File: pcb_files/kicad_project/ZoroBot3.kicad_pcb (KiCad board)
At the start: 2 copper layers, 67.6 x 110.7 mm, 175 parts, among them Q1 NMOS, Q2 AON7423, Q3 ST-1KL3A, Q4 ST-1KL3A, Q5 ST-1KL3A, Q6 ST-1KL3A, U1 MPU-6500, U2 MPU-6500, Y1 Crystal_GND24

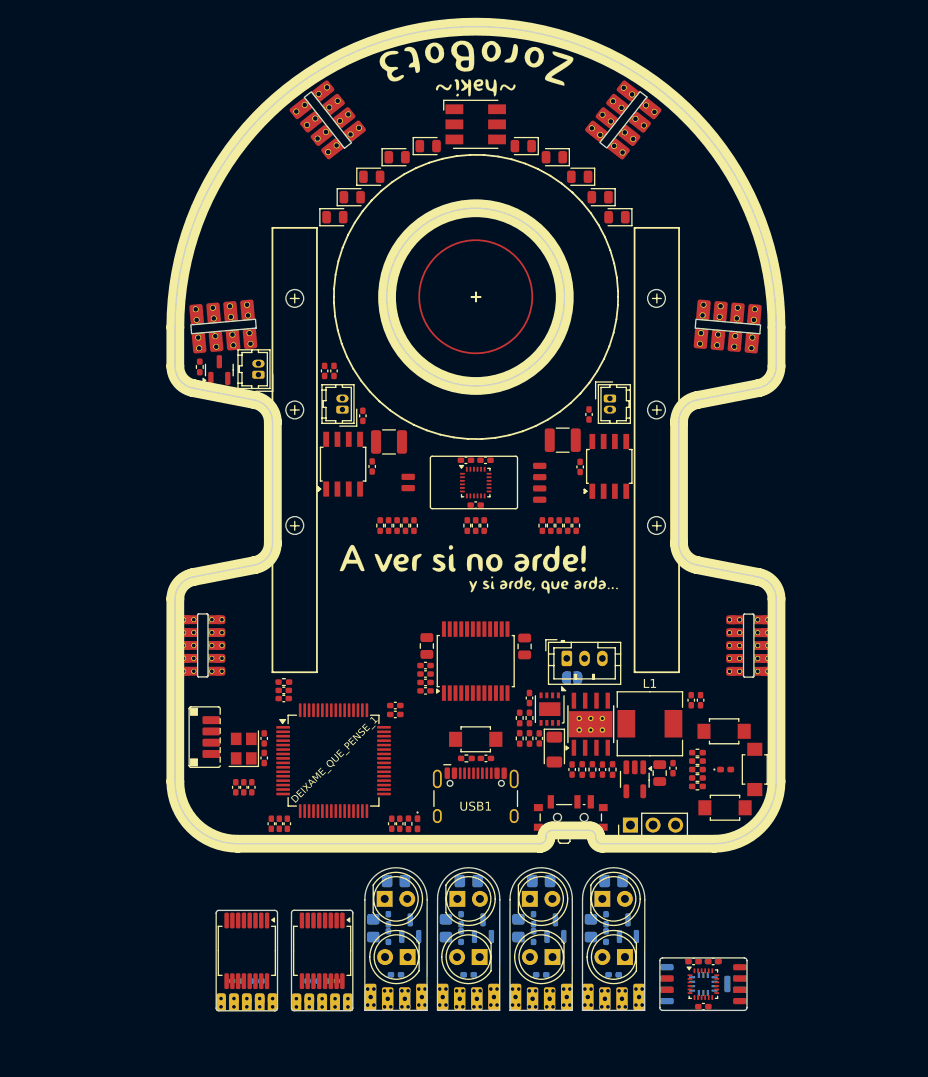
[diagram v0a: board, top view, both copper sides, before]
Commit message: Finaliza el diseño de la PCB de ZoroBot3 Rebuild y añade gerbers y BOM
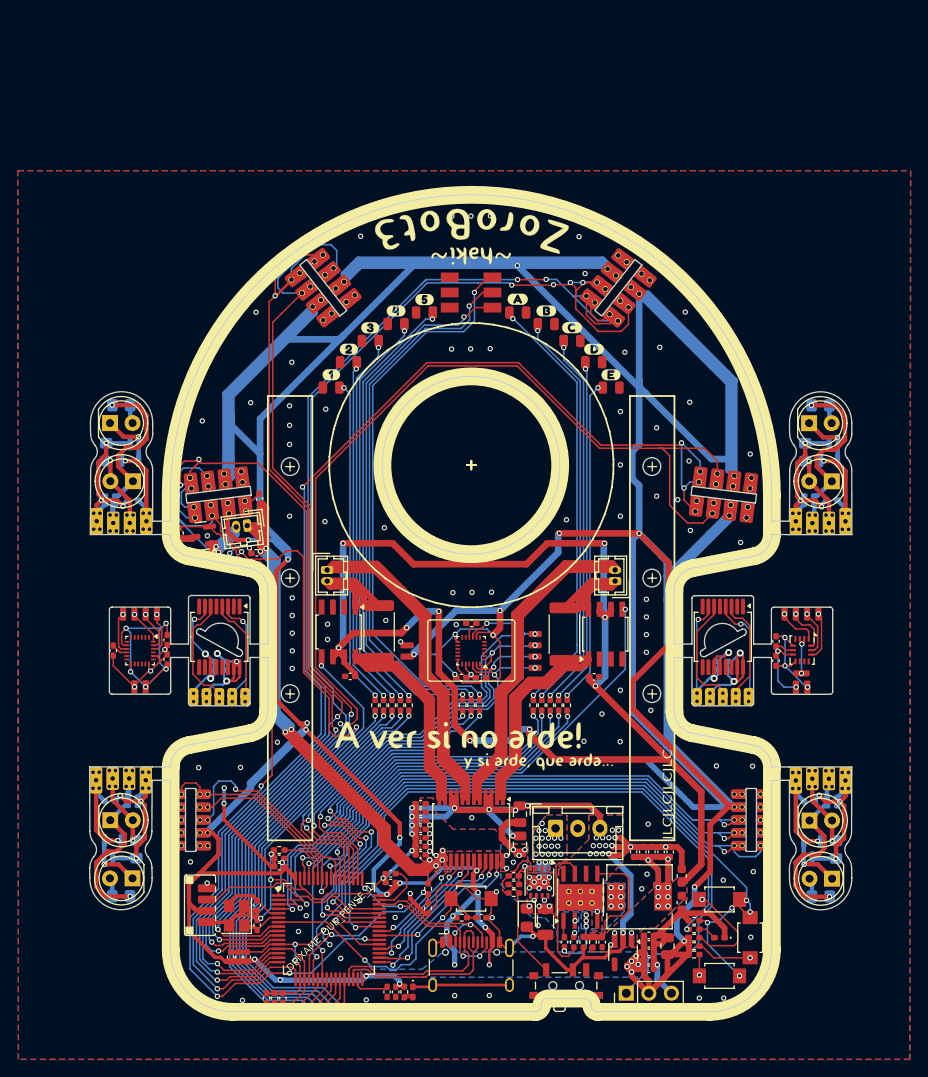
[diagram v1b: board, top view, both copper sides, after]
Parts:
- removed C14, C16: 0.1uF, Capacitor_SMD:C_0402_1005Metric_Pad0.74x0.62mm_HandSolder
- added C41: 10uF, Capacitor_SMD:C_0402_1005Metric_Pad0.74x0.62mm_HandSolder, F.Cu at (144.9, 119.4)
- added C42: 10uF, Capacitor_SMD:C_0402_1005Metric_Pad0.74x0.62mm_HandSolder, F.Cu at (144.9, 120.4)
- added C43: 10uF, Capacitor_SMD:C_0402_1005Metric_Pad0.74x0.62mm_HandSolder, F.Cu at (144.9, 121.4)
- added C44: 10uF, Capacitor_SMD:C_0402_1005Metric_Pad0.74x0.62mm_HandSolder, F.Cu at (170.6, 137.1)
- added C45: 10uF, Capacitor_SMD:C_0402_1005Metric_Pad0.74x0.62mm_HandSolder, F.Cu at (170.6, 135.2)
- added C46: 10uF, Capacitor_SMD:C_0402_1005Metric_Pad0.74x0.62mm_HandSolder, F.Cu at (170.6, 136.2)
- added C47: 10uF, Capacitor_SMD:C_0402_1005Metric_Pad0.74x0.62mm_HandSolder, F.Cu at (173.0, 124.9)
- added C48: 10uF, Capacitor_SMD:C_0402_1005Metric_Pad0.74x0.62mm_HandSolder, F.Cu at (170.9, 124.9)
- added C49: 10uF, Capacitor_SMD:C_0402_1005Metric_Pad0.74x0.62mm_HandSolder, F.Cu at (172.0, 124.9)
- added C50: 10uF, Capacitor_SMD:C_0402_1005Metric_Pad0.74x0.62mm_HandSolder, F.Cu at (168.9, 124.9)
- added C51: 10uF, Capacitor_SMD:C_0402_1005Metric_Pad0.74x0.62mm_HandSolder, F.Cu at (169.9, 124.9)
- added C52: 10uF, Capacitor_SMD:C_0402_1005Metric_Pad0.74x0.62mm_HandSolder, F.Cu at (170.6, 138.1)
- added kibuzzard-6779A98A: G***, kibuzzard-6779A98A, B.Cu at (110.8, 99.0)
- added kibuzzard-6779A9B1: G***, kibuzzard-6779A9B1, B.Cu at (185.3, 98.9)
- added kibuzzard-677A7C8F: G***, kibuzzard-677A7C8F, F.Cu at (155.8, 62.7)
- added kibuzzard-677A7C9A: G***, kibuzzard-677A7C9A, F.Cu at (159.0, 64.0)
- added kibuzzard-677A7CA3: G***, kibuzzard-677A7CA3, F.Cu at (161.9, 65.9)
- added kibuzzard-677A7CAF: G***, kibuzzard-677A7CAF, F.Cu at (164.4, 68.3)
- added kibuzzard-677A7CBB: G***, kibuzzard-677A7CBB, F.Cu at (166.3, 71.2)
- added kibuzzard-677A7D71: G***, kibuzzard-677A7D71, F.Cu at (136.8, 68.3)
- added kibuzzard-677A7D7B: G***, kibuzzard-677A7D7B, F.Cu at (139.2, 65.9)
- added kibuzzard-677A7D86: G***, kibuzzard-677A7D86, F.Cu at (142.1, 64.0)
- added kibuzzard-677A7E2E: G***, kibuzzard-677A7E2E, F.Cu at (134.8, 71.2)
- added kibuzzard-677A7E3B: G***, kibuzzard-677A7E3B, F.Cu at (145.3, 62.7)
- AS5145B_D1, AS5145B_I1: footprint Package_SO:SSOP-16_5.3x6.2mm_P0.65mm -> custom_footprints:Encoder_AS5145B
- BATT1: footprint Connector_JST:JST_PH_B3B-PH-K_1x03_P2.00mm_Vertical -> Connector_JST:JST_XH_B3B-XH-A_1x03_P2.50mm_Vertical
- C37, C38, DATA_MPU2, JP3, LSM6DSR1, POWER_MPU3: moved to F.Cu
- CR4, CR7: footprint Capacitor_SMD:C_0402_1005Metric_Pad0.74x0.62mm_HandSolder -> Capacitor_SMD:C_0603_1608Metric
- CR6: value 0.1uF -> 47uF; footprint Capacitor_SMD:C_0402_1005Metric_Pad0.74x0.62mm_HandSolder -> Capacitor_SMD:C_1206_3216Metric
- D13: footprint Diode_SMD:D_1206_3216Metric -> Diode_SMD:D_0805_2012Metric_Pad1.15x1.40mm_HandSolder
- MOSFET-N1, MOSFET-N2, MOSFET-N3, MOSFET-N4: value AO3401 -> AO3400 (A09T)
- R12, R13: footprint Resistor_SMD:R_1210_3225Metric -> Resistor_SMD:R_2512_6332Metric
- moved DATA_MPU3 79.3 mm to (113.3, 98.1), turned to 90 degrees
- moved C40 77.5 mm to (110.3, 102.2), turned to 90 degrees
- moved POWER_MPU3 75.3 mm to (113.3, 106.3), turned to 90 degrees
- moved U2 73.7 mm to (113.3, 102.2), turned to -90 degrees
- moved C39 71.3 mm to (116.4, 101.0), turned to 90 degrees
- moved C36 68.3 mm to (116.4, 103.2), turned to -90 degrees
- moved C33 65.4 mm to (178.9, 103.4), turned to 180 degrees
- moved AS5145B_D1 64.2 mm to (178.9, 100.7)
- moved ENC_D_CONN1 63.6 mm to (178.9, 106.3)
- moved C32 63.1 mm to (178.9, 104.4)
- moved RS9 62.5 mm to (188.2, 79.9)
- moved CONN_SEN_PA_I1 62.3 mm to (111.2, 87.8)
- moved MOSFET-N2 62.2 mm to (112.2, 79.9)
- moved LED_IR3 62.1 mm to (188.6, 76.6)
- moved RS7 62.1 mm to (189.9, 74.6)
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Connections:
- AD8418AWBZ_2 pad 1: /SHUNT_MI -> /MOT_I-
- AD8418AWBZ_2 pad 8: /MOT_I+ -> /SHUNT_MI
- C36 pad 1: /Giroscopio/GND_MPU -> /Giroscopio/GND_MPU_A
- C36 pad 2: /Giroscopio/3.3_MPU -> /Giroscopio/3.3_MPU_A
- C37 pad 1: /Giroscopio/GND_MPU -> /Giroscopio/GND_MPU_B
- C37 pad 2: /Giroscopio/3.3_MPU -> /Giroscopio/3.3_MPU_B
- C38 pad 1: /Giroscopio/GND_MPU -> /Giroscopio/GND_MPU_B
- C38 pad 2: /Giroscopio/3.3_MPU -> /Giroscopio/3.3_MPU_B
- C39 pad 1: /Giroscopio/GND_MPU -> /Giroscopio/GND_MPU_A
- C39 pad 2: /Giroscopio/3.3_MPU -> /Giroscopio/3.3_MPU_A
- C40 pad 1: /Giroscopio/GND_MPU -> /Giroscopio/GND_MPU_A
- DATA_MPU2 pad 1: /Giroscopio/SPI_MISO_CONN -> /Giroscopio/SPI_MISO_CONN_B
- DATA_MPU2 pad 2: /Giroscopio/SPI_MOSI_CONN -> /Giroscopio/SPI_MOSI_CONN_B
- DATA_MPU2 pad 3: /Giroscopio/SPI_SCK_CONN -> /Giroscopio/SPI_SCK_CONN_B
- DATA_MPU2 pad 4: /Giroscopio/SPI_NSS_CONN -> /Giroscopio/SPI_NSS_CONN_B
- DATA_MPU3 pad 1: /Giroscopio/SPI_MISO_CONN -> /Giroscopio/SPI_MISO_CONN_A
- DATA_MPU3 pad 2: /Giroscopio/SPI_MOSI_CONN -> /Giroscopio/SPI_MOSI_CONN_A
- DATA_MPU3 pad 3: /Giroscopio/SPI_SCK_CONN -> /Giroscopio/SPI_SCK_CONN_A
- DATA_MPU3 pad 4: /Giroscopio/SPI_NSS_CONN -> /Giroscopio/SPI_NSS_CONN_A
- DEIXAME_QUE_PENSE_1 pad 54: /ENC_2_I -> /ENC_D_I
- DEIXAME_QUE_PENSE_1 pad 55: /ENC_1_I -> /ENC_I_I
- DEIXAME_QUE_PENSE_1 pad 56: /ENC_2_B -> /ENC_D_B
- DEIXAME_QUE_PENSE_1 pad 57: /ENC_2_A -> /ENC_D_A
- DEIXAME_QUE_PENSE_1 pad 58: /ENC_1_B -> /ENC_I_B
- DEIXAME_QUE_PENSE_1 pad 59: /ENC_1_A -> /ENC_I_A
- ENC_D1 pad 3: /ENC_1_A -> /ENC_D_I
- ENC_D1 pad 4: /ENC_1_B -> /ENC_D_A
- ENC_D1 pad 5: /ENC_1_I -> /ENC_D_B
- ENC_D_CONN1 pad 3: /Encoders/ENC_D_A_CONN -> /Encoders/ENC_D_I_CONN
- ENC_D_CONN1 pad 4: /Encoders/ENC_D_B_CONN -> /Encoders/ENC_D_A_CONN
- ENC_D_CONN1 pad 5: /Encoders/ENC_D_I_CONN -> /Encoders/ENC_D_B_CONN
- ENC_I1 pad 3: /ENC_2_A -> /ENC_I_I
- ENC_I1 pad 4: /ENC_2_B -> /ENC_I_A
- ENC_I1 pad 5: /ENC_2_I -> /ENC_I_B
- ENC_I_CONN1 pad 3: /Encoders/ENC_I_A_CONN -> /Encoders/ENC_I_I_CONN
- ENC_I_CONN1 pad 4: /Encoders/ENC_I_B_CONN -> /Encoders/ENC_I_A_CONN
- ENC_I_CONN1 pad 5: /Encoders/ENC_I_I_CONN -> /Encoders/ENC_I_B_CONN
- LSM6DSR1 pad 1: /Giroscopio/SPI_MISO_CONN -> /Giroscopio/SPI_MISO_CONN_B
- LSM6DSR1 pad 12: /Giroscopio/SPI_NSS_CONN -> /Giroscopio/SPI_NSS_CONN_B
- LSM6DSR1 pad 13: /Giroscopio/SPI_SCK_CONN -> /Giroscopio/SPI_SCK_CONN_B
- LSM6DSR1 pad 14: /Giroscopio/SPI_MOSI_CONN -> /Giroscopio/SPI_MOSI_CONN_B
- LSM6DSR1 pad 5: /Giroscopio/3.3_MPU -> /Giroscopio/3.3_MPU_B
- LSM6DSR1 pad 6: /Giroscopio/GND_MPU -> /Giroscopio/GND_MPU_B
- LSM6DSR1 pad 7: /Giroscopio/GND_MPU -> /Giroscopio/GND_MPU_B
- LSM6DSR1 pad 8: /Giroscopio/3.3_MPU -> /Giroscopio/3.3_MPU_B
- MOSFET-N1 pad 1: /Sensores/EMI_PA_D_CONN -> Net-(LED_IR1-K)
- MOSFET-N1 pad 2: /Sensores/GND_D -> /Sensores/EMI_PA_D_CONN
- MOSFET-N1 pad 3: Net-(LED_IR1-K) -> /Sensores/GND_D
- MOSFET-N2 pad 1: /Sensores/EMI_PA_I_CONN -> Net-(LED_IR2-K)
- MOSFET-N2 pad 2: /Sensores/GND_I -> /Sensores/EMI_PA_I_CONN
- MOSFET-N2 pad 3: Net-(LED_IR2-K) -> /Sensores/GND_I
- MOSFET-N3 pad 1: /Sensores/EMI_FRONT_D_CONN -> Net-(LED_IR3-K)
- MOSFET-N3 pad 2: /Sensores/GND_FD -> /Sensores/EMI_FRONT_D_CONN
- MOSFET-N3 pad 3: Net-(LED_IR3-K) -> /Sensores/GND_FD
- MOSFET-N4 pad 1: /Sensores/EMI_FRONT_I_CONN -> Net-(LED_IR4-K)
- MOSFET-N4 pad 2: /Sensores/GND_FI -> /Sensores/EMI_FRONT_I_CONN
- MOSFET-N4 pad 3: Net-(LED_IR4-K) -> /Sensores/GND_FI
- PH1 pad 1: /BATT -> /SHUNT_MD
- PH1 pad 10: /MOT_I_PWM -> GND
- PH1 pad 11: /BATT -> /SHUNT_MI
- PH1 pad 12: /BATT -> /SHUNT_MI
- PH1 pad 13: /SHUNT_MI -> /BATT
- PH1 pad 14: /SHUNT_MI -> /BATT
- PH1 pad 15: GND -> /MOT_I_PWM
- PH1 pad 16: GND -> /MOT_I_B
- PH1 pad 17: /MOT_I- -> /MOT_I_A
- PH1 pad 18: /MOT_I- -> GND
- PH1 pad 19: /MOT_D- -> +3V3
- PH1 pad 2: /MOT_D_PWM -> /SHUNT_MD
- PH1 pad 20: /MOT_D- -> +3V3
- PH1 pad 21: GND -> /MOT_D_B
- PH1 pad 22: GND -> /MOT_D_A
- PH1 pad 23: /SHUNT_MD -> /MOT_D_PWM
- PH1 pad 24: /SHUNT_MD -> /BATT
- PH1 pad 3: /MOT_D_A -> GND
- PH1 pad 4: /MOT_D_B -> GND
- PH1 pad 5: +3V3 -> /MOT_D-
- PH1 pad 6: +3V3 -> /MOT_D-
- PH1 pad 7: GND -> /MOT_I+
- PH1 pad 8: /MOT_I_A -> /MOT_I+
- PH1 pad 9: /MOT_I_B -> GND
- POWER_MPU2 pad 1: /Giroscopio/GND_MPU -> /Giroscopio/GND_MPU_B
- POWER_MPU2 pad 2: /Giroscopio/3.3_MPU -> /Giroscopio/3.3_MPU_B
- POWER_MPU3 pad 1: /Giroscopio/GND_MPU -> /Giroscopio/GND_MPU_A
- POWER_MPU3 pad 2: /Giroscopio/3.3_MPU -> /Giroscopio/3.3_MPU_A
- POWER_SWITCH1 pad 1: unconnected-(POWER_SWITCH1-A-Pad1) -> Net-(POWER_SWITCH1-A)
- POWER_SWITCH1 pad 3: Net-(POWER_SWITCH1-C) -> unconnected-(POWER_SWITCH1-C-Pad3)
- R13 pad 1: /MOT_I+ -> /MOT_I-
- R27 pad 1: Net-(POWER_SWITCH1-C) -> Net-(POWER_SWITCH1-A)
- R28 pad 1: Net-(POWER_SWITCH1-C) -> Net-(POWER_SWITCH1-A)
- U2 pad 13: /Giroscopio/3.3_MPU -> /Giroscopio/3.3_MPU_A
- U2 pad 18: /Giroscopio/GND_MPU -> /Giroscopio/GND_MPU_A
- U2 pad 20: /Giroscopio/GND_MPU -> /Giroscopio/GND_MPU_A
- U2 pad 22: /Giroscopio/SPI_NSS_CONN -> /Giroscopio/SPI_NSS_CONN_A
- U2 pad 23: /Giroscopio/SPI_SCK_CONN -> /Giroscopio/SPI_SCK_CONN_A
- U2 pad 24: /Giroscopio/SPI_MOSI_CONN -> /Giroscopio/SPI_MOSI_CONN_A
- U2 pad 8: /Giroscopio/3.3_MPU -> /Giroscopio/3.3_MPU_A
- U2 pad 9: /Giroscopio/SPI_MISO_CONN -> /Giroscopio/SPI_MISO_CONN_A
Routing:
- net +3V3: track 0.00 -> 804.2 mm, vias 0 -> 35
- net GND: track 0.00 -> 289.1 mm, vias 0 -> 130
- net +5V: track 0.00 -> 164.6 mm, vias 0 -> 20
- net /EMI_FRONT_D: track 0.00 -> 142.2 mm, vias 0 -> 4
- net /SEN_FRONT_D: track 0.00 -> 141.4 mm, vias 0 -> 2
- net /EMI_PA_I: track 0.00 -> 136.3 mm, vias 0 -> 3
- net /SEN_PA_I: track 0.00 -> 132.6 mm, vias 0 -> 5
- net /BATT: track 0.00 -> 117.9 mm, vias 0 -> 34
- net /EMI_PA_D: track 0.00 -> 117.1 mm, vias 0 -> 3
- net /SEN_PA_D: track 0.00 -> 106.3 mm, vias 0 -> 2
- net /EMI_FRONT_I: track 0.00 -> 101.2 mm, vias 0 -> 4
- net /SEN_FRONT_I: track 0.00 -> 99.5 mm, vias 0 -> 3
- net /MENU_ANALOG: track 0.00 -> 88.6 mm, vias 0 -> 6
- net /MOT_S_PWM: track 0.00 -> 86.8 mm, vias 0 -> 4
- net /AUX_PIN: track 0.00 -> 83.2 mm, vias 0 -> 1
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- added copper zone on B.Cu, net +3V3
- added copper zone on B.Cu, net +5V
- added copper zone on F.Cu, net +5V
- added copper zone on B.Cu, net /BATT
- added copper zone on F.Cu, net /BATT
- added copper zone on B.Cu, net /LIPO+
- added copper zone on F.Cu, net /LIPO+
- added copper zone on B.Cu, net GND
- added copper zone on F.Cu, net GND
- added copper zone on B.Cu, net Net-(DC-DC1-SW)
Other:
- board size 67.6 x 110.7 mm -> 85.8 x 91.9 mm
- board text added: "JLCJLCJLCJLC"
